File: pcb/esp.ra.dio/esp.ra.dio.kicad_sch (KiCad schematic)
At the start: 45 parts, among them J1 A, J10 UART, J2 B, J3 C, J4 D, J5 START, J6 SELECT, J7 JOY, J8 USB_B_Micro, J9 BATTERY, Q1 BSS84, SW1 POWER, SW2 RESET, SW3 BOOT, U2 VCC, U3 RT9080-33GJ5, U4 SN74LV165APWRG3

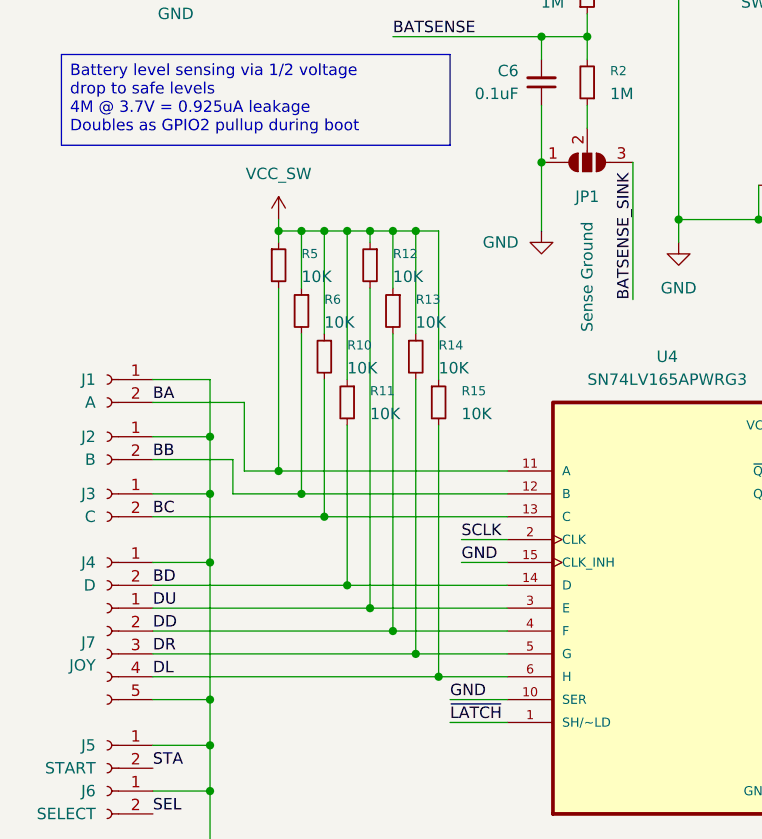
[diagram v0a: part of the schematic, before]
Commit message: Horrible routing job done
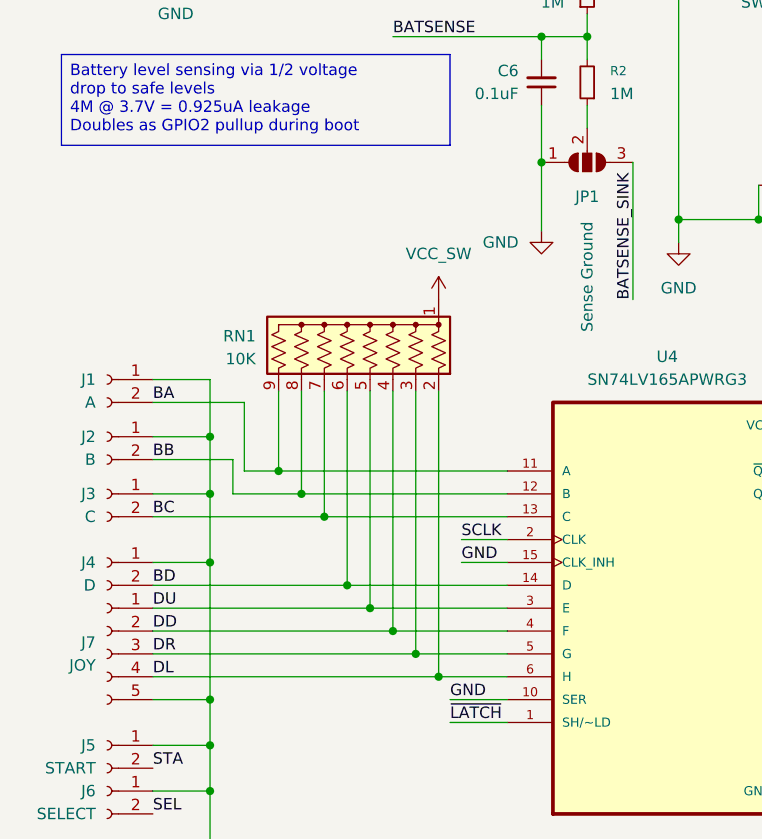
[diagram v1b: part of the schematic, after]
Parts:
- removed R10, R11, R12, R13, R14, R15, R5, R6: 10K, Resistor_SMD:R_0805_2012Metric_Pad1.20x1.40mm_HandSolder, symbol Device:R_Small
- added RN1: 10K, RN:RN, symbol Device:R_Network08_US
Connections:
- net BA: now also RN1.9 (R8)
- net BB: now also RN1.8 (R7)
- net BC: now also RN1.7 (R6)
- net BD: now also RN1.6 (R5)
- net DD: now also RN1.4 (R3)
- net DL: now also RN1.2 (R1)
- net DR: now also RN1.3 (R2)
- net DU: now also RN1.5 (R4)
- net VCC_SW: now also RN1.1 (common)
